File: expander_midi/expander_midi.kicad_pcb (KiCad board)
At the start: 2 copper layers, 70.4 x 128.5 mm, 44 parts, among them J1_BACK PinHeader_2x06_P2.54mm_Vertic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, J1_FRONT PinSocket_2x06_P2.54mm_Vertic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, J2_BACK PinHeader_1x06_P2.54mm_Vertic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, J2_FRONT PinHeader_1x06_P2.54mm_Vertic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, U1 LD1117

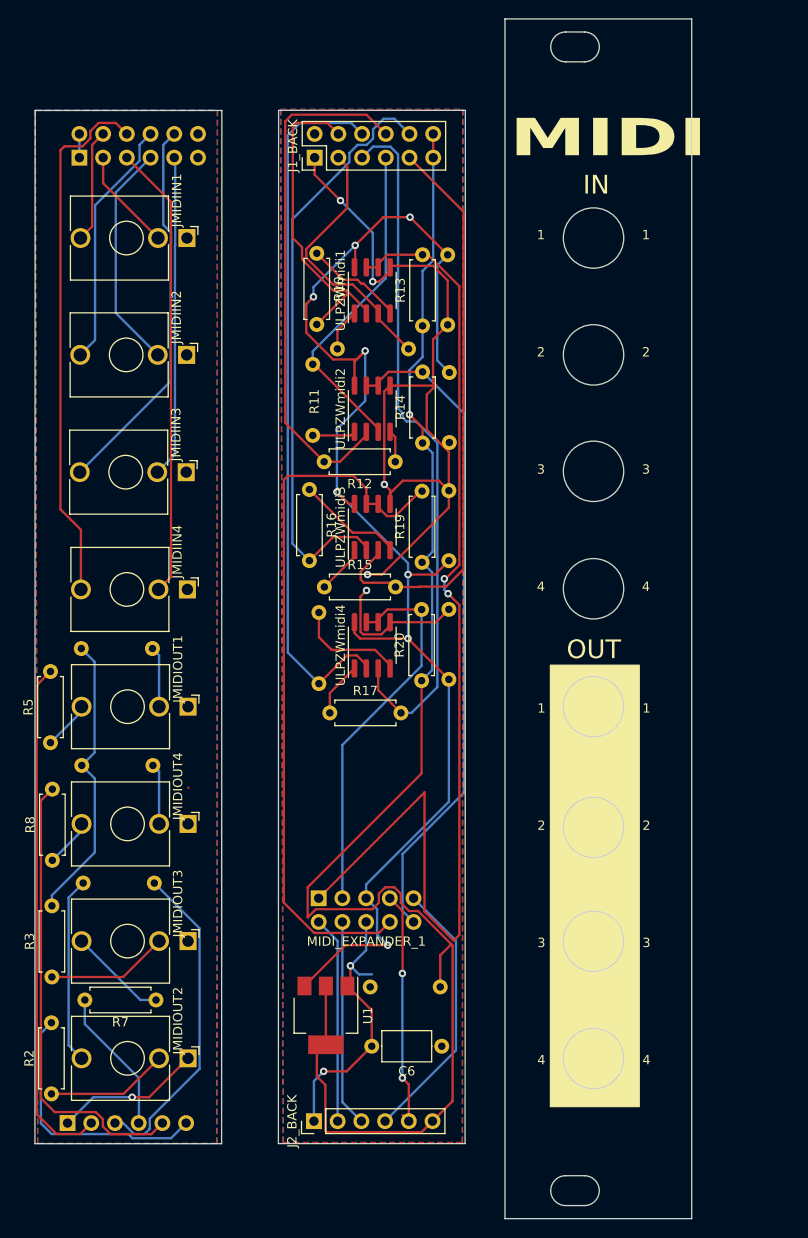
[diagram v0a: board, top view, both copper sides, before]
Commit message: laid out quite nicely now i think
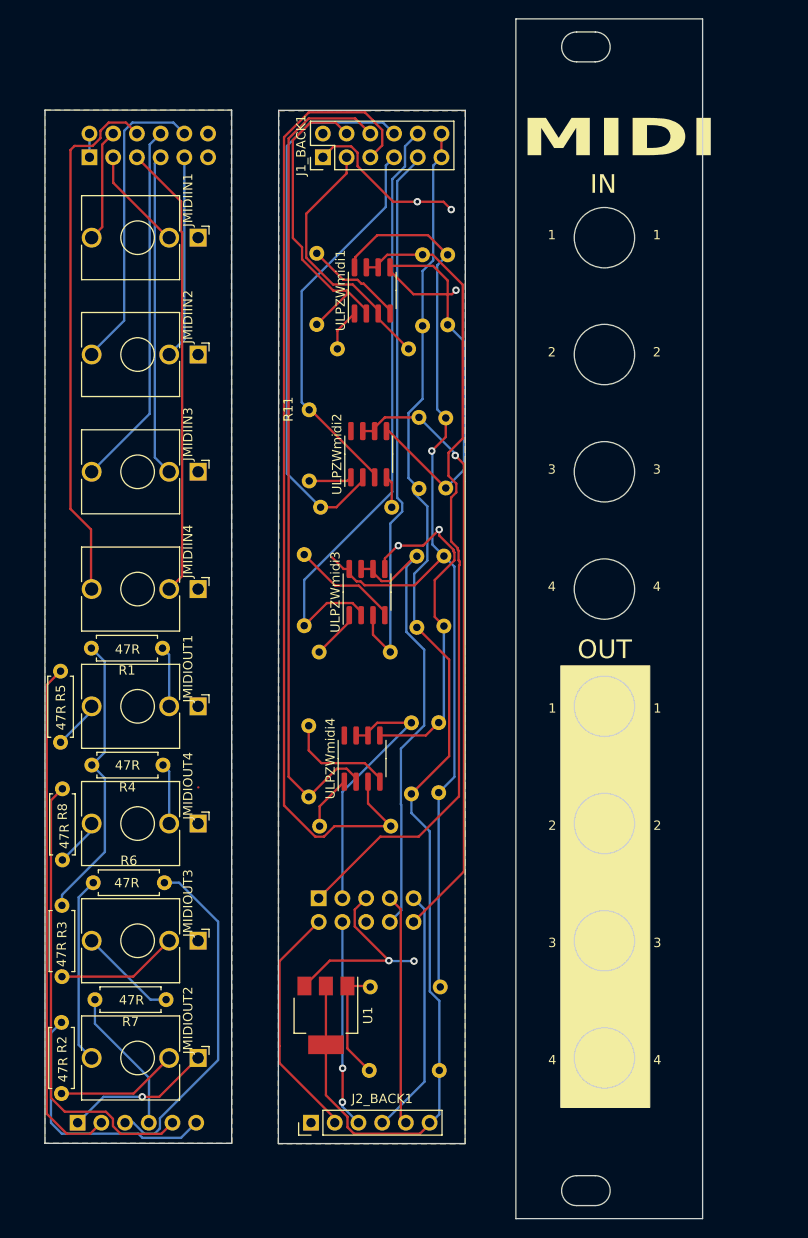
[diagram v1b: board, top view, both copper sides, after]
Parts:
- C2: value 100nF -> 100n
- C4: value 100n -> 100nF
- C6, R10, R12, R13, R14, R15, R16, R17, R19, R20: moved to B.Cu
- J1_BACK1: renamed from J1_BACK; value PinHeader_2x06_P2.54mm_Vertical -> Conn_02x06_Odd_Even
- J1_FRONT1: renamed from J1_FRONT; value PinSocket_2x06_P2.54mm_Vertical -> Conn_02x06_Odd_Even
- J2_BACK1: renamed from J2_BACK; value PinHeader_1x06_P2.54mm_Vertical -> Conn_01x06_Pin
- J2_FRONT1: renamed from J2_FRONT; value PinHeader_1x06_P2.54mm_Vertical -> Conn_01x06_Socket; footprint Connector_PinHeader_2.54mm:PinHeader_1x06_P2.54mm_Vertical -> Connector_PinSocket_2.54mm:PinSocket_1x06_P2.54mm_Vertical
- R1, R4, R6: moved to F.Cu
- moved C4 54.6 mm to (217.4, 152.9), turned to 180 degrees
- moved C6 52.5 mm to (217.9, 97.8), turned to -90 degrees
- moved C3 12.2 mm to (217.3, 123.2)
- moved R17 12.2 mm to (204.6, 126.8)
- moved R18 12.2 mm to (203.4, 116.0)
- moved ULPZWmidi4 12.2 mm to (209.1, 119.5)
- moved R20 12.2 mm to (214.4, 123.3)
- moved R15 6.99 mm to (204.5, 108.1)
- moved R16 6.99 mm to (202.9, 97.7)
- moved R19 6.99 mm to (215.0, 105.5)
- moved ULPZWmidi3 6.99 mm to (209.7, 101.7)
- moved C5 4.89 mm to (218.1, 83.1)
- moved R11 4.89 mm to (203.5, 89.8)
- moved R12 4.89 mm to (212.3, 92.6)
- moved R14 4.89 mm to (215.2, 90.6)
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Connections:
- C2 pad 1: +3V3 -> +5V
- C4 pad 1: +5V -> +3V3
- J1_BACK1 pad 10: MIDI_IN_T_4 -> MIDI_IN_T_4_BACK
- J1_BACK1 pad 3: MIDI_IN_R_1 -> MIDI_IN_R_1_BACK
- J1_BACK1 pad 4: MIDI_IN_T_1 -> MIDI_IN_T_1_BACK
- J1_BACK1 pad 5: MIDI_IN_R_2 -> MIDI_IN_R_2_BACK
- J1_BACK1 pad 6: MIDI_IN_T_2 -> MIDI_IN_T_2_BACK
- J1_BACK1 pad 7: MIDI_IN_R_3 -> MIDI_IN_R_3_BACK
- J1_BACK1 pad 8: MIDI_IN_T_3 -> MIDI_IN_T_3_BACK
- J1_BACK1 pad 9: MIDI_IN_R_4 -> MIDI_IN_R_4_BACK
- J1_FRONT1 pad 10: MIDI_IN_T_4 -> MIDI_IN_T_4_FRONT
- J1_FRONT1 pad 3: MIDI_IN_R_1 -> MIDI_IN_R_1_FRONT
- J1_FRONT1 pad 4: MIDI_IN_T_1 -> MIDI_IN_T_1_FRONT
- J1_FRONT1 pad 5: MIDI_IN_R_2 -> MIDI_IN_R_2_FRONT
- J1_FRONT1 pad 6: MIDI_IN_T_2 -> MIDI_IN_T_2_FRONT
- J1_FRONT1 pad 7: MIDI_IN_R_3 -> MIDI_IN_R_3_FRONT
- J1_FRONT1 pad 8: MIDI_IN_T_3 -> MIDI_IN_T_3_FRONT
- J1_FRONT1 pad 9: MIDI_IN_R_4 -> MIDI_IN_R_4_FRONT
- J2_FRONT1 pad 2: MIDI_1_TX -> MIDI_1_TX_FRONT
- J2_FRONT1 pad 3: MIDI_2_TX -> MIDI_2_TX_FRONT
- J2_FRONT1 pad 4: MIDI_3_TX -> MIDI_3_TX_FRONT
- J2_FRONT1 pad 5: MIDI_4_TX -> MIDI_4_TX_FRONT
- JMIDIIN1 pad R: MIDI_IN_R_1 -> MIDI_IN_R_1_FRONT
- JMIDIIN1 pad T: MIDI_IN_T_1 -> MIDI_IN_T_1_FRONT
- JMIDIIN2 pad R: MIDI_IN_R_3 -> MIDI_IN_R_4_FRONT
- JMIDIIN2 pad T: MIDI_IN_T_3 -> MIDI_IN_T_4_FRONT
- JMIDIIN3 pad R: MIDI_IN_R_4 -> MIDI_IN_R_3_FRONT
- JMIDIIN3 pad T: MIDI_IN_T_4 -> MIDI_IN_T_3_FRONT
- JMIDIIN4 pad R: MIDI_IN_R_2 -> MIDI_IN_R_2_FRONT
- JMIDIIN4 pad T: MIDI_IN_T_2 -> MIDI_IN_T_2_FRONT
- R10 pad 2: MIDI_IN_T_1 -> MIDI_IN_T_1_BACK
- R11 pad 2: MIDI_IN_R_3 -> MIDI_IN_R_3_BACK
- R12 pad 2: MIDI_IN_T_3 -> MIDI_IN_T_3_BACK
- R15 pad 2: MIDI_IN_R_4 -> MIDI_IN_R_4_BACK
- R16 pad 2: MIDI_IN_T_4 -> MIDI_IN_T_4_BACK
- R17 pad 2: MIDI_IN_R_2 -> MIDI_IN_R_2_BACK
- R18 pad 2: MIDI_IN_T_2 -> MIDI_IN_T_2_BACK
- R5 pad 2: MIDI_1_TX -> MIDI_1_TX_FRONT
- R6 pad 2: MIDI_2_TX -> MIDI_2_TX_FRONT
- R7 pad 2: MIDI_3_TX -> MIDI_3_TX_FRONT
- R8 pad 2: MIDI_4_TX -> MIDI_4_TX_FRONT
- R9 pad 2: MIDI_IN_R_1 -> MIDI_IN_R_1_BACK
- ULPZWmidi1 pad 2: MIDI_IN_T_1 -> MIDI_IN_T_1_BACK
- ULPZWmidi1 pad 3: MIDI_IN_R_1 -> MIDI_IN_R_1_BACK
- ULPZWmidi2 pad 2: MIDI_IN_T_3 -> MIDI_IN_T_3_BACK
- ULPZWmidi2 pad 3: MIDI_IN_R_3 -> MIDI_IN_R_3_BACK
- ULPZWmidi3 pad 2: MIDI_IN_T_4 -> MIDI_IN_T_4_BACK
- ULPZWmidi3 pad 3: MIDI_IN_R_4 -> MIDI_IN_R_4_BACK
- ULPZWmidi4 pad 2: MIDI_IN_T_2 -> MIDI_IN_T_2_BACK
- ULPZWmidi4 pad 3: MIDI_IN_R_2 -> MIDI_IN_R_2_BACK
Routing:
- net MIDI_IN_T_2: track 133.1 -> 0.00 mm
- net MIDI_IN_R_2: track 123.7 -> 0.00 mm
- net MIDI_IN_R_2_BACK: track 0.00 -> 106.5 mm
- net MIDI_IN_T_4: track 104.8 -> 0.00 mm
- net MIDI_IN_R_4: track 95.8 -> 0.00 mm
- net MIDI_IN_T_2_BACK: track 0.00 -> 88.5 mm
- net MIDI_IN_T_3: track 82.6 -> 0.00 mm
- net MIDI_IN_T_4_BACK: track 0.00 -> 65.2 mm
- net MIDI_IN_R_3: track 59.6 -> 0.00 mm
- net MIDI_IN_R_4_BACK: track 0.00 -> 59.0 mm
- net MIDI_IN_T_3_BACK: track 0.00 -> 58.9 mm
- net MIDI_IN_T_2_FRONT: track 0.00 -> 57.1 mm
- net MIDI_1_TX_FRONT: track 0.00 -> 55.2 mm
- net MIDI_1_TX: track 77.4 -> 25.2 mm
- net MIDI_4_TX: track 74.9 -> 24.8 mm, vias 2 -> 0
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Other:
- outline, holes or cut-outs redrawn
- board text added: "!!!NOT POWER!!!"
